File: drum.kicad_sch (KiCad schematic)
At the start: 39 parts, among them J101 Cortex, J102 DX07S016JA3, SW101 SKSG, SW102 SKSG, U101 ATSAMD51J, U102 TPS78433QWDRBRQ1, Y101 32k768

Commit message: Update Library
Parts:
- C101: symbol V2_Device:C_0603_10u -> V2_Capacitor:0603_10u
- C102, C103, C104, C105, C106: symbol V2_Device:C_0603_0u1 -> V2_Capacitor:0603_0u1
- C107, C108: symbol V2_Device:C_0603_18p -> V2_Capacitor:0603_18p
- C109, C110: symbol V2_Device:C_0805_10u -> V2_Capacitor:0805_10u
- D101: symbol V2_Device:LED_0603_Orange -> V2_LED:0603_Orange
- INFO102: value (none) -> ~
- R101: symbol V2_Device:R_0603_330R -> V2_Resistor:0603_330R
- R102, R103: symbol V2_Device:R_0603_5k1 -> V2_Resistor:0603_5k1
- R104: symbol V2_Device:R_0603_100k -> V2_Resistor:0603_100k
- Y101: symbol V2_Device:Crystal_3.2x1.5_32k768 -> V2_Crystal:3.2x1.5_32k768
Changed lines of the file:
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@@
 	)
 	(symbol
-		(lib_id "V2_Device:C_0603_0u1")
+		(lib_id "V2_Capacitor:0603_0u1")
 		(at 109.22 24.13 0)
 		(unit 1)
@@
 		(at 240.03 170.18 0)
 		(unit 1)
-		(exclude_from_sim no)
+		(exclude_from_sim yes)
 		(in_bom no)
 		(on_board yes)
@@
 	)
 	(symbol
-		(lib_id "V2_Device:LED_0603_Orange")
+		(lib_id "V2_LED:0603_Orange")
 		(at 129.54 86.36 0)
 		(mirror y)
@@
 	)
 	(symbol
-		(lib_id "V2_Device:R_0603_5k1")
+		(lib_id "V2_Resistor:0603_5k1")
 		(at 203.2 119.38 90)
 		(unit 1)
@@
 		(at 227.33 180.34 0)
 		(unit 1)
-		(exclude_from_sim no)
+		(exclude_from_sim yes)
 		(in_bom no)
 		(on_board yes)
@@
 	)
 	(symbol
-		(lib_id "V2_Device:C_0805_10u")
+		(lib_id "V2_Capacitor:0805_10u")
 		(at 55.88 180.34 0)
 		(unit 1)
@@
 	)
 	(symbol
-		(lib_id "V2_Device:C_0603_0u1")
+		(lib_id "V2_Capacitor:0603_0u1")
 		(at 119.38 24.13 0)
 		(unit 1)
@@
 		(at 240.03 165.1 0)
 		(unit 1)
-		(exclude_from_sim no)
+		(exclude_from_sim yes)
 		(in_bom no)
 		(on_board yes)
@@
 			)
 		)
-		(property "Value" ""
+		(property "Value" "~"
 			(at 248.92 182.88 0)
 			(effects
@@
 	)
 	(symbol
-		(lib_id "V2_Device:C_0805_10u")
+		(lib_id "V2_Capacitor:0805_10u")
 		(at 30.48 180.34 0)
 		(unit 1)
@@
 	)
 	(symbol
-		(lib_id "V2_Device:Crystal_3.2x1.5_32k768")
+		(lib_id "V2_Crystal:3.2x1.5_32k768")
 		(at 24.13 43.18 0)
 		(unit 1)
@@
 	)
 	(symbol
-		(lib_id "V2_Device:C_0603_18p")
+		(lib_id "V2_Capacitor:0603_18p")
 		(at 26.67 46.99 0)
 		(unit 1)
@@
 	)
 	(symbol
-		(lib_id "V2_Device:C_0603_10u")
+		(lib_id "V2_Capacitor:0603_10u")
 		(at 57.15 24.13 0)
 		(unit 1)
@@
 	)
 	(symbol
-		(lib_id "V2_Device:C_0603_18p")
+		(lib_id "V2_Capacitor:0603_18p")
 		(at 21.59 46.99 0)
 		(unit 1)
@@
 	)
 	(symbol
-		(lib_id "V2_Device:R_0603_330R")
+		(lib_id "V2_Resistor:0603_330R")
 		(at 138.43 86.36 90)
 		(unit 1)
@@
 	)
 	(symbol
-		(lib_id "V2_Device:C_0603_0u1")
+		(lib_id "V2_Capacitor:0603_0u1")
 		(at 99.06 24.13 0)
 		(unit 1)
@@
 	)
 	(symbol
-		(lib_id "V2_Device:C_0603_0u1")
+		(lib_id "V2_Capacitor:0603_0u1")
 		(at 78.74 24.13 0)
 		(unit 1)
@@
 	)
 	(symbol
-		(lib_id "V2_Device:R_0603_5k1")
+		(lib_id "V2_Resistor:0603_5k1")
 		(at 203.2 116.84 90)
 		(unit 1)
@@
 	)
 	(symbol
-		(lib_id "V2_Device:C_0603_0u1")
+		(lib_id "V2_Capacitor:0603_0u1")
 		(at 88.9 24.13 0)
 		(unit 1)
@@
 	)
 	(symbol
-		(lib_id "V2_Device:R_0603_100k")
+		(lib_id "V2_Resistor:0603_100k")
 		(at 50.8 121.92 90)
 		(unit 1)

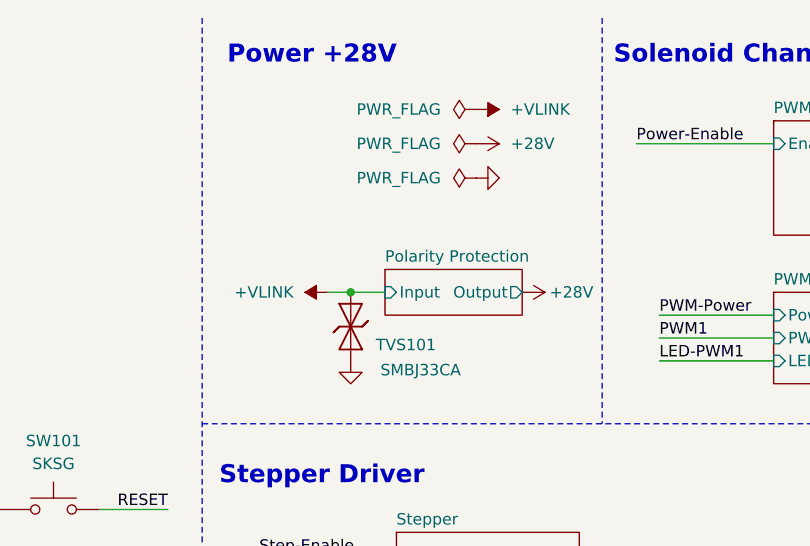
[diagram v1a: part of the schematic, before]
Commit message: Refresh
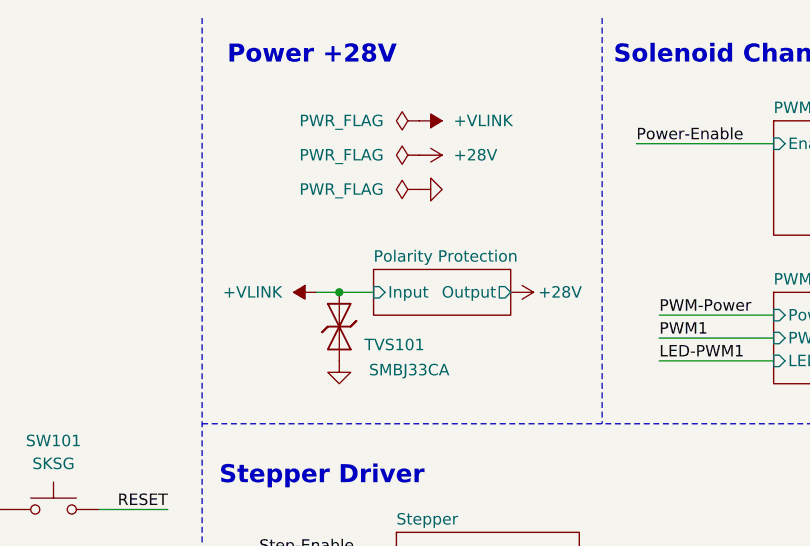
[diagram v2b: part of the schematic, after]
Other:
- moved on the sheet: TVS101
